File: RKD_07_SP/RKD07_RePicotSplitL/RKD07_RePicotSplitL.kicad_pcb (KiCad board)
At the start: 2 copper layers, 36.9 x 81 mm, 16 parts, among them J101 Conn_01x24, J102 Conn_01x06, J151 Conn_01x06, J152 Qwiic_RA, J153 6P6C, J154 Conn_01x02_Socket, J155 Conn_01x08, J１03 Conn_01x06, U101 Pico

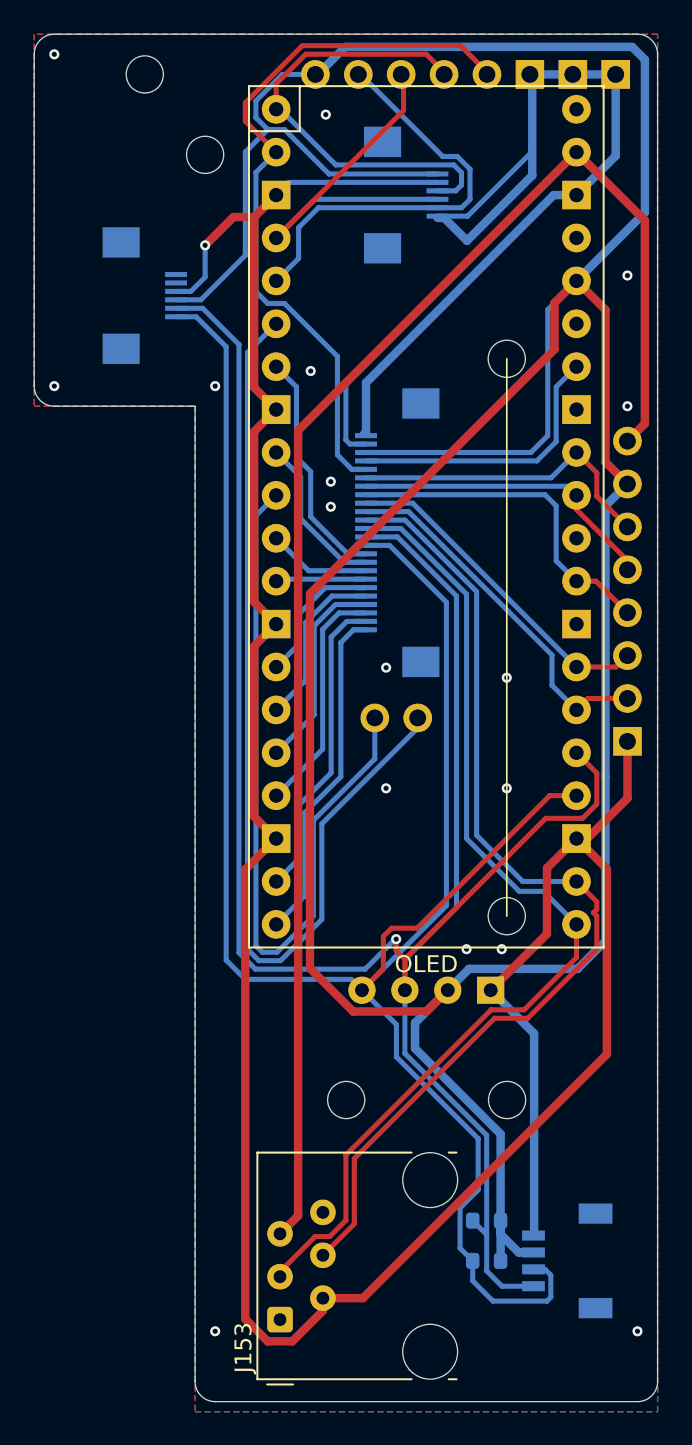
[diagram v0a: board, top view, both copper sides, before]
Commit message: Combine
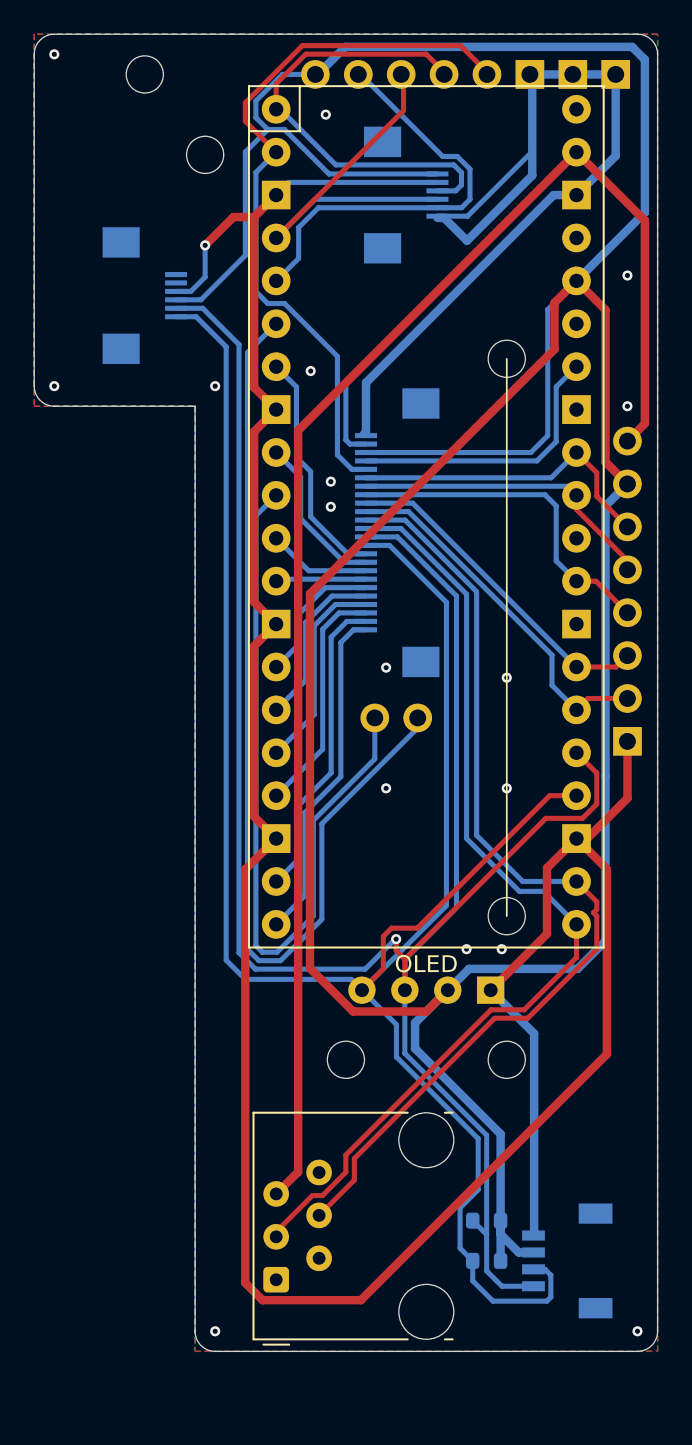
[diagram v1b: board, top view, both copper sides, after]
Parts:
- moved Point1 2.38 mm to (164.3, 58.3)
- moved J153 2.37 mm to (155.4, 101.1)
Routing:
- net GND_L: track 223.9 -> 220.2 mm
- net COL6_GP16_L: track 60.4 -> 58.0 mm
- net VCC_L: track 114.5 -> 112.2 mm
- net COL7_GP17_L: track 60.4 -> 58.2 mm
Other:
- board size 36.9 x 81 mm -> 36.9 x 78 mm
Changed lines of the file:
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@@
 	(footprint "Rikkodo_FootPrint:rkd_Guard_Screw_Hall"
 		(layer "F.Cu")
-		(at 164.325122 60.72188 -90)
+		(at 164.306145 58.34048 -90)
 		(property "Reference" "Point1"
 			(at 7 8.1 90)
@@
 	(footprint "Connector_RJ:RJ12_Amphenol_54601-x06_Horizontal"
 		(layer "F.Cu")
-		(at 155.643144 103.490072 90)
+		(at 155.416112 101.128672 90)
 		(descr "RJ12 6P6C horizontal socket, plastic body, tab down, https://cdn.amphenol-icc.com/media/wysiwyg/files/drawing/c-bmj-0082.pdf")
 		(tags "RJ12 connector")
@@
 			(at -1.66 -2.16 90)
 			(layer "F.SilkS")
+			(hide yes)
 			(effects
 				(font
@@
 	(gr_line
 		(start 150.614205 49.410979)
-		(end 150.614188 107.15625)
+		(end 150.614189 104.173827)
 		(stroke
 			(width 0.05)
@@
 	)
 	(gr_arc
-		(start 177.998629 107.156227)
-		(mid 177.649905 107.998131)
-		(end 176.808004 108.346875)
+		(start 177.998629 104.179577)
+		(mid 177.649905 105.021481)
+		(end 176.808004 105.370225)
 		(stroke
 			(width 0.05)
@@
 	)
 	(gr_line
-		(start 151.804795 108.346875)
-		(end 176.807961 108.346875)
+		(start 151.804795 105.370225)
+		(end 176.807961 105.370225)
 		(stroke
 			(width 0.05)
@@
 	)
 	(gr_arc
-		(start 151.804795 108.346875)
-		(mid 150.962893 107.998148)
-		(end 150.614147 107.15625)
+		(start 151.804795 105.370225)
+		(mid 150.962893 105.021498)
+		(end 150.614147 104.1796)
 		(stroke
 			(width 0.05)
@@
 	)
 	(gr_line
-		(start 177.998587 107.1662)
+		(start 177.998588 104.16972)
 		(end 177.998601 28.575023)
 		(stroke
@@
 	)
 	(segment
-		(start 157.722952 98.569072)
-		(end 158.585624 98.569072)
+		(start 155.416112 98.28748)
+		(end 157.560704 96.142888)
 		(width 0.3)
 		(layer "F.Cu")
@@
 	)
 	(segment
-		(start 155.643144 100.950072)
-		(end 155.643144 100.64888)
+		(start 155.416112 98.588672)
+		(end 155.416112 98.28748)
 		(width 0.3)
 		(layer "F.Cu")
@@
 	)
 	(segment
-		(start 170.101668 85.1454)
-		(end 173.196374 82.050694)
+		(start 159.54375 94.762226)
+		(end 159.54375 93.742024)
 		(width 0.3)
 		(layer "F.Cu")
@@
 	)
 	(segment
-		(start 173.196374 82.050694)
-		(end 173.196374 80.0894)
+		(start 170.101668 85.1454)
+		(end 173.196374 82.050694)
 		(width 0.3)
 		(layer "F.Cu")
@@
 	)
 	(segment
-		(start 158.585624 98.569072)
-		(end 159.54375 97.610946)
+		(start 173.196374 82.050694)
+		(end 173.196374 80.0894)
 		(width 0.3)
 		(layer "F.Cu")
@@
 	)
 	(segment
-		(start 159.54375 97.610946)
-		(end 159.54375 93.742024)
+		(start 157.560704 96.142888)
+		(end 158.163088 96.142888)
 		(width 0.3)
 		(layer "F.Cu")
@@
 	)
 	(segment
-		(start 155.643144 100.64888)
-		(end 157.722952 98.569072)
+		(start 158.163088 96.142888)
+		(end 159.54375 94.762226)
 		(width 0.3)
 		(layer "F.Cu")
@@
 	)
 	(segment
-		(start 160.04475 97.818466)
-		(end 160.04475 93.949544)
-		(width 0.3)
-		(layer "F.Cu")
-		(net 9)
-	)
-	(segment
 		(start 170.309189 85.6464)
 		(end 174.397374 81.558214)
@@
 	)
 	(segment
-		(start 158.183144 99.680072)
-		(end 160.04475 97.818466)
-		(width 0.3)
-		(layer "F.Cu")
-		(net 9)
-	)
-	(segment
 		(start 174.397374 79.205751)
 		(end 174.397374 78.7504)
@@
 	)
 	(segment
+		(start 160.04475 95.230034)
+		(end 157.956112 97.318672)
+		(width 0.3)
+		(layer "F.Cu")
+		(net 9)
+	)
+	(segment
+		(start 160.04475 93.949544)
+		(end 160.04475 95.230034)
+		(width 0.3)
+		(layer "F.Cu")
+		(net 9)
+	)
+	(segment
 		(start 174.204285 79.39884)
 		(end 174.397374 79.205751)
@@
 	)
 	(segment
+		(start 153.590496 101.321348)
+		(end 154.60882 102.339672)
+		(width 0.5)
+		(layer "F.Cu")
+		(net 10)
+	)
+	(segment
+		(start 160.430162 102.339672)
+		(end 174.998374 87.77146)
+		(width 0.5)
+		(layer "F.Cu")
+		(net 10)
+	)
+	(segment
+		(start 174.998374 76.8114)
+		(end 173.196374 75.0094)
+		(width 0.5)
+		(layer "F.Cu")
+		(net 10)
+	)
+	(segment
 		(start 171.45 80.650774)
 		(end 168.116374 83.9844)
@@
 	)
 	(segment
+		(start 174.998374 87.77146)
+		(end 174.998374 76.8114)
+		(width 0.5)
+		(layer "F.Cu")
+		(net 10)
+	)
+	(segment
 		(start 155.416374 62.3094)
 		(end 154.115374 63.6104)
@@
 	)
 	(segment
-		(start 173.196374 75.0094)
-		(end 171.45 76.755774)
+		(start 155.416374 75.0094)
+		(end 153.590496 76.835278)
 		(width 0.5)
 		(layer "F.Cu")
@@
 	)
 	(segment
-		(start 160.549762 102.220072)
-		(end 158.183144 102.220072)
+		(start 173.196374 75.0094)
+		(end 171.45 76.755774)
 		(width 0.5)
 		(layer "F.Cu")
@@
 	)
 	(segment
-		(start 155.416374 75.0094)
-		(end 153.590496 76.835278)
-		(width 0.5)
-		(layer "F.Cu")
-		(net 10)
-	)
-	(segment
 		(start 155.416374 49.6094)
 		(end 154.115374 48.3084)
@@
 	)
 	(segment
-		(start 174.998374 76.8114)
-		(end 174.998374 87.77146)
-		(width 0.5)
-		(layer "F.Cu")
-		(net 10)
-	)
-	(segment
-		(start 154.90978 104.775)
-		(end 156.376508 104.775)
+		(start 154.60882 102.339672)
+		(end 160.430162 102.339672)
 		(width 0.5)
 		(layer "F.Cu")
@@
 	)
 	(segment
-		(start 158.183144 102.968364)
-		(end 158.183144 102.220072)
+		(start 153.590496 76.835278)
+		(end 153.590496 101.321348)
 		(width 0.5)
 		(layer "F.Cu")
@@
 	)
 	(segment
-		(start 156.376508 104.775)
-		(end 158.183144 102.968364)
-		(width 0.5)
-		(layer "F.Cu")
-		(net 10)
-	)
-	(segment
 		(start 154.115374 63.6104)
 		(end 154.115374 73.7084)
@@
 	)
 	(segment
-		(start 153.590496 76.835278)
-		(end 153.590496 103.455716)
-		(width 0.5)
-		(layer "F.Cu")
-		(net 10)
-	)
-	(segment
-		(start 153.590496 103.455716)
-		(end 154.90978 104.775)
-		(width 0.5)
-		(layer "F.Cu")
-		(net 10)
-	)
-	(segment
 		(start 173.196374 75.0094)
 		(end 173.831225 75.0094)
@@
 		(net 10)
 	)
-	(segment
-		(start 174.998374 87.77146)
-		(end 160.549762 102.220072)
-		(width 0.5)
-		(layer "F.Cu")
-		(net 10)
-	)
-	(segment
-		(start 173.196374 75.0094)
-		(end 174.998374 76.8114)
-		(width 0.5)
-		(layer "F.Cu")
-		(net 10)
-	)
 	(via
 		(at 151.80456 104.1796)
@@
 	)
 	(segment
-		(start 155.643144 98.410072)
-		(end 156.717374 97.335842)
+		(start 156.717374 94.74741)
+		(end 156.717374 50.8484)
 		(width 0.5)
 		(layer "F.Cu")
@@
 	)
 	(segment
-		(start 156.717374 97.335842)
-		(end 156.717374 50.8484)
+		(start 177.247597 38.420623)
+		(end 173.196374 34.3694)
 		(width 0.5)
 		(layer "F.Cu")
@@
 	)
 	(segment
-		(start 177.247597 38.420623)
-		(end 173.196374 34.3694)
+		(start 155.416112 96.048672)
+		(end 156.717374 94.74741)
 		(width 0.5)
 		(layer "F.Cu")
@@
 		(polygon
 			(pts
-				(xy 141.089181 27.384398) (xy 141.089181 49.410979) (xy 150.614189 49.410979) (xy 150.614189 108.942276)
-				(xy 177.998587 108.942276) (xy 177.998587 27.384398)
+				(xy 141.089181 27.384398) (xy 141.089181 49.410979) (xy 150.614189 49.410979) (xy 150.614189 105.370404)
+				(xy 177.998587 105.370404) (xy 177.998587 27.384398)
 			)
 		)
